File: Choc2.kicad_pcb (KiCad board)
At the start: 2 copper layers, 40 x 100 mm, 19 parts, among them J1 Conn_01x02, J4 Conn_01x03, SW1 SW_PUSH, SW2 SW_PUSH, SW3 SW_PUSH, SW4 SW_PUSH, SW5 SW_PUSH, SW6 SW_PUSH, SW7 SW_PUSH, U1 xiao-th

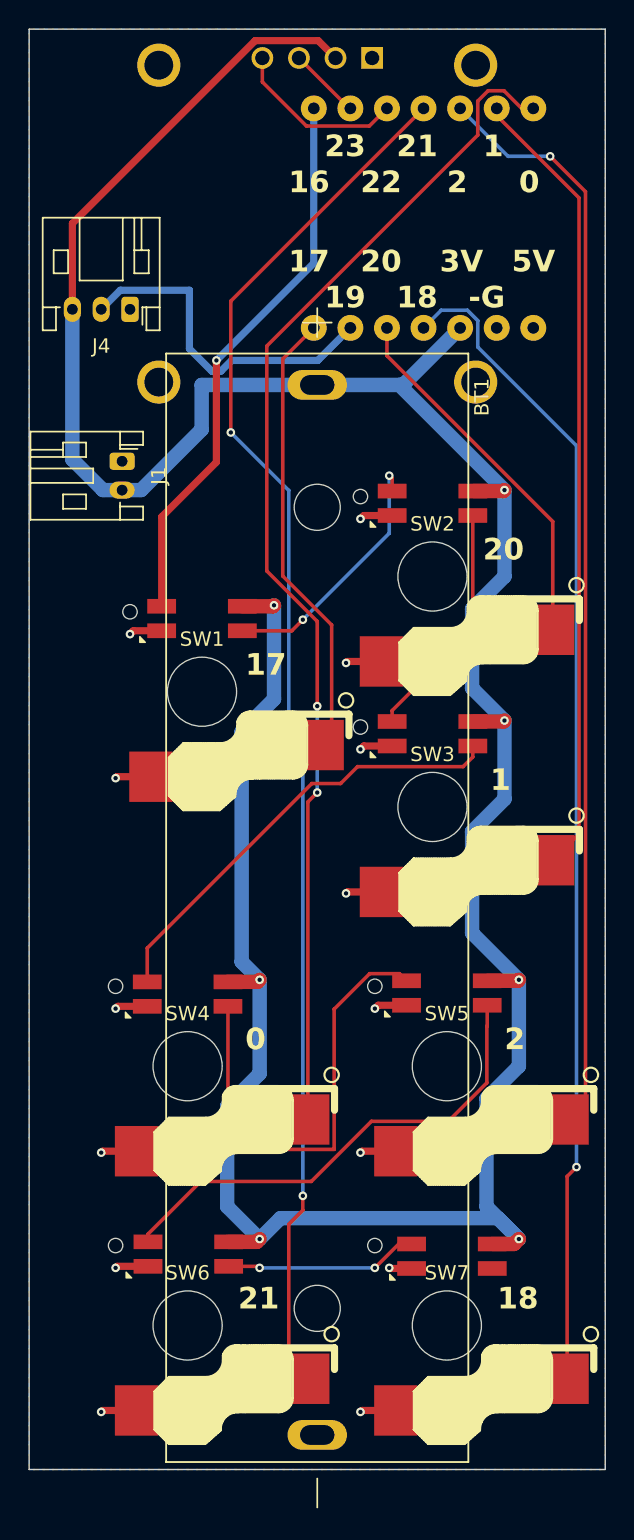
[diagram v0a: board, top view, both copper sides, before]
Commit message: chipSocket
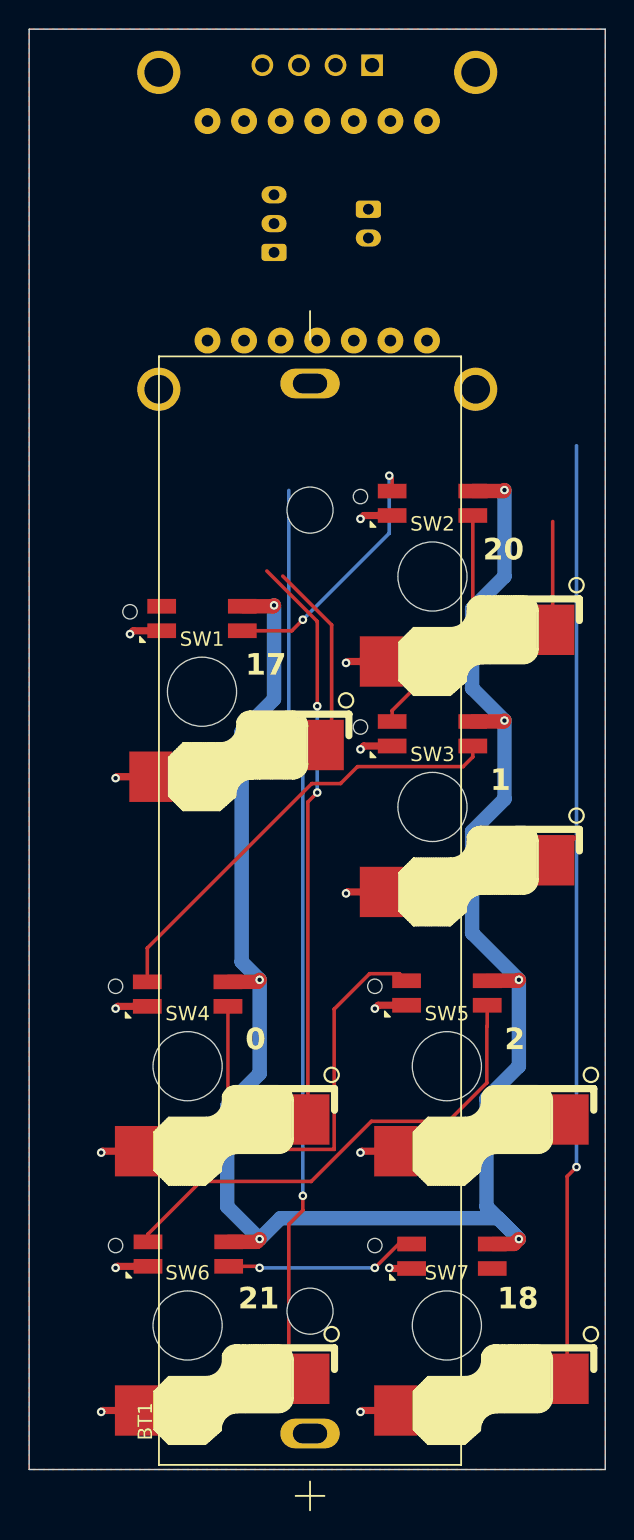
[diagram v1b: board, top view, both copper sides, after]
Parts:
- J1, J4: moved to B.Cu
- U1: moved to F.Cu
- moved J1 24.5 mm to (73.5, 62.5)
- moved J4 10.8 mm to (67.0, 65.5), turned to 90 degrees
- moved U1 7.43 mm to (70.0, 64.0), turned to -90 degrees
- moved BT1 0.54 mm to (69.5, 111.2), turned to 90 degrees
- moved OL1 0.50 mm to (70.0, 64.0)
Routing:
- net VCC: track 224.9 -> 139.9 mm
- net SW5: track 76.0 -> 1.80 mm, vias 1 -> 0
- net SW3: track 55.3 -> 2.58 mm
- net SW4: track 83.2 -> 39.8 mm
- net LED: track 38.9 -> 0.00 mm, vias 1 -> 0
- net SW6: track 96.8 -> 63.0 mm, vias 2 -> 1
- net LED2: track 23.8 -> 0.00 mm
- net SW2: track 25.7 -> 7.52 mm
- net SW1: track 31.5 -> 13.4 mm
- net SW7: track 81.1 -> 65.1 mm
- net SDA: track 12.1 -> 0.00 mm
- net SCL: track 5.48 -> 0.00 mm
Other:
- board text removed: "-G"
- board text removed: "16"
- board text removed: "19"
- board text removed: "22"
- board text removed: "23"
- board text removed: "3V"
- board text removed: "5V"
